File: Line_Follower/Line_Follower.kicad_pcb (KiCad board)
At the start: 2 copper layers, 95.5 x 93.5 mm, 20 parts, among them J1 Battery terminal, J10 Motor_B, J11 8-Channel IR Array, J9 Motor_A, SW1 Slide Switch, SW3 Mode, SW6 Calibration, U1 ESP32-DEVKITC, U2 LM2596 Buck Converter, U3 TB6612FNG_MD

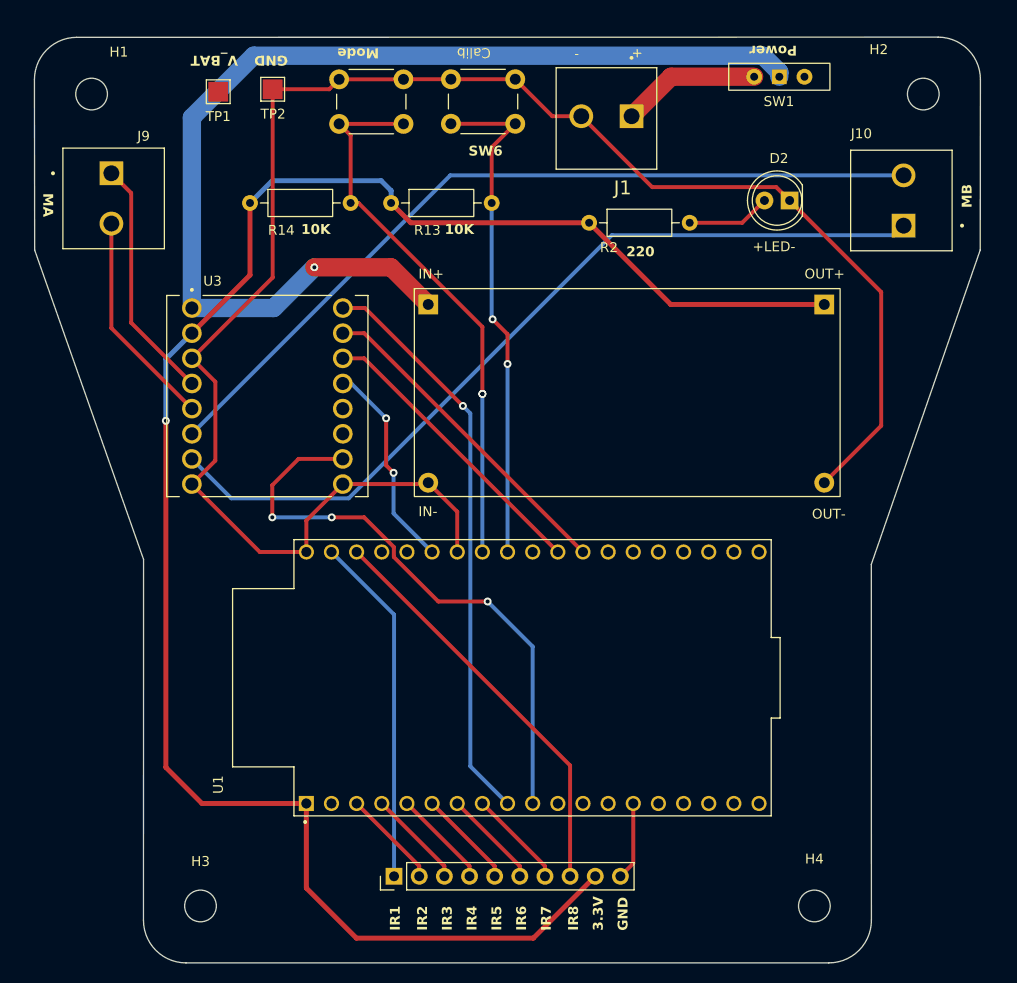
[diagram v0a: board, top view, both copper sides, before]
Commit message: Routing done
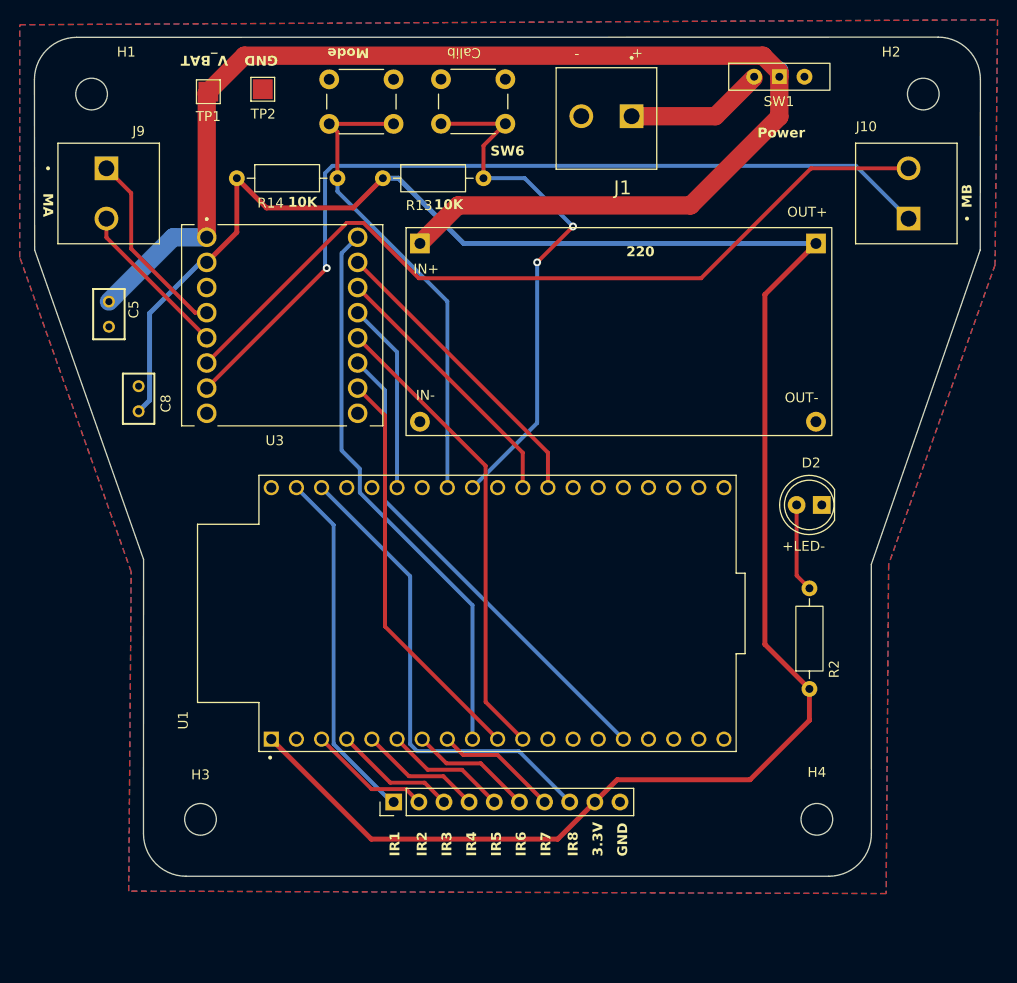
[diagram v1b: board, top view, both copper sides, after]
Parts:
- added C5: 100nF, Capacitors:C320C, F.Cu at (113.0, 65.0)
- added C8: 100nF, Capacitors:C320C, F.Cu at (102.0, 59.5)
- moved R2 52.1 mm to (176.8, 95.8), turned to 90 degrees
- moved D2 30.9 mm to (178.0, 77.2)
- moved H4 8.75 mm to (177.5, 109.0)
- moved H3 8.75 mm to (115.2, 109.0)
- moved J11 7.50 mm to (134.8, 107.2)
- moved U1 7.40 mm to (145.2, 88.2)
- moved U3 7.31 mm to (123.5, 59.1)
- moved U2 6.22 mm to (136.0, 70.2)
- moved R14 2.83 mm to (118.9, 44.2)
- moved R13 2.63 mm to (133.7, 44.2)
- moved SW3 1.00 mm to (128.2, 34.3)
- moved SW6 1.00 mm to (139.5, 34.2)
- moved TP1 1.00 mm to (116.0, 35.5)
- moved TP2 1.00 mm to (121.5, 35.3)
- moved J10 0.87 mm to (186.8, 48.3)
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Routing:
- net GND: track 185.4 -> 0.02 mm
- net BIN2: track 0.00 -> 49.1 mm
- net BIN1: track 0.00 -> 47.4 mm
- net VBAT+: track 109.4 -> 134.0 mm, vias 1 -> 0
- net 3V3: track 183.6 -> 207.4 mm, vias 1 -> 0
- net PWMB: track 59.6 -> 41.3 mm, vias 3 -> 0
- net MODE: track 56.2 -> 48.2 mm, vias 2 -> 0
- net IR8: track 41.7 -> 48.1 mm
- net MA2: track 22.1 -> 16.2 mm
- net MA1: track 24.6 -> 19.5 mm
- net MB1: track 84.9 -> 88.3 mm, vias 0 -> 1
- net CAL: track 51.4 -> 54.6 mm
- net AIN2: track 33.4 -> 30.7 mm
- net AIN1: track 29.8 -> 27.1 mm
- net IR6: track 9.97 -> 12.5 mm
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- added copper zone on B.Cu, net GND
- added copper zone on F.Cu, net GND
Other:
- board size 95.5 x 93.5 mm -> 95.5 x 84.7 mm
